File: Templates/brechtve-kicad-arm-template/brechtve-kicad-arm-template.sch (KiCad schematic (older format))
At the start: 16 parts, among them J1 DebugHeader_Cortex-M_SWD_UART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, J2 DebugHeader_Cortex-M_JTAG_10p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, J3 DebugHeader_UART_4p, SW1 SW_Push

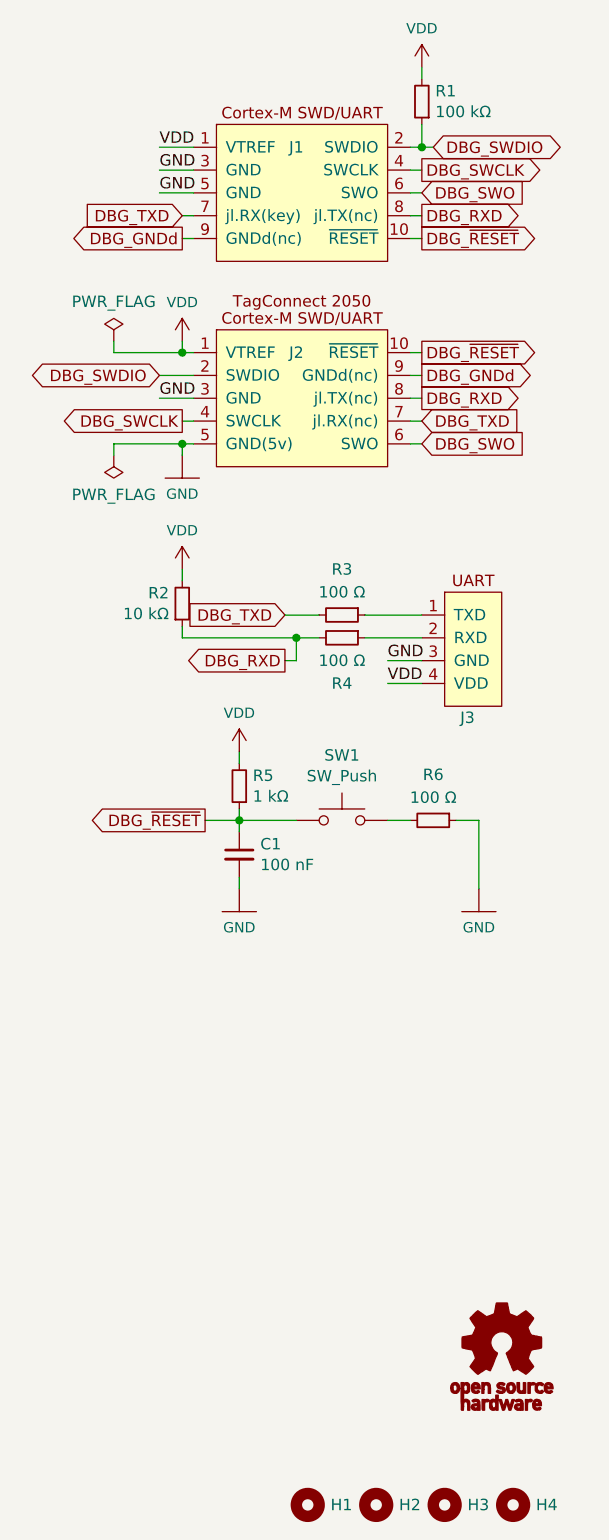
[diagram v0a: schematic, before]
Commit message: Modified schematic
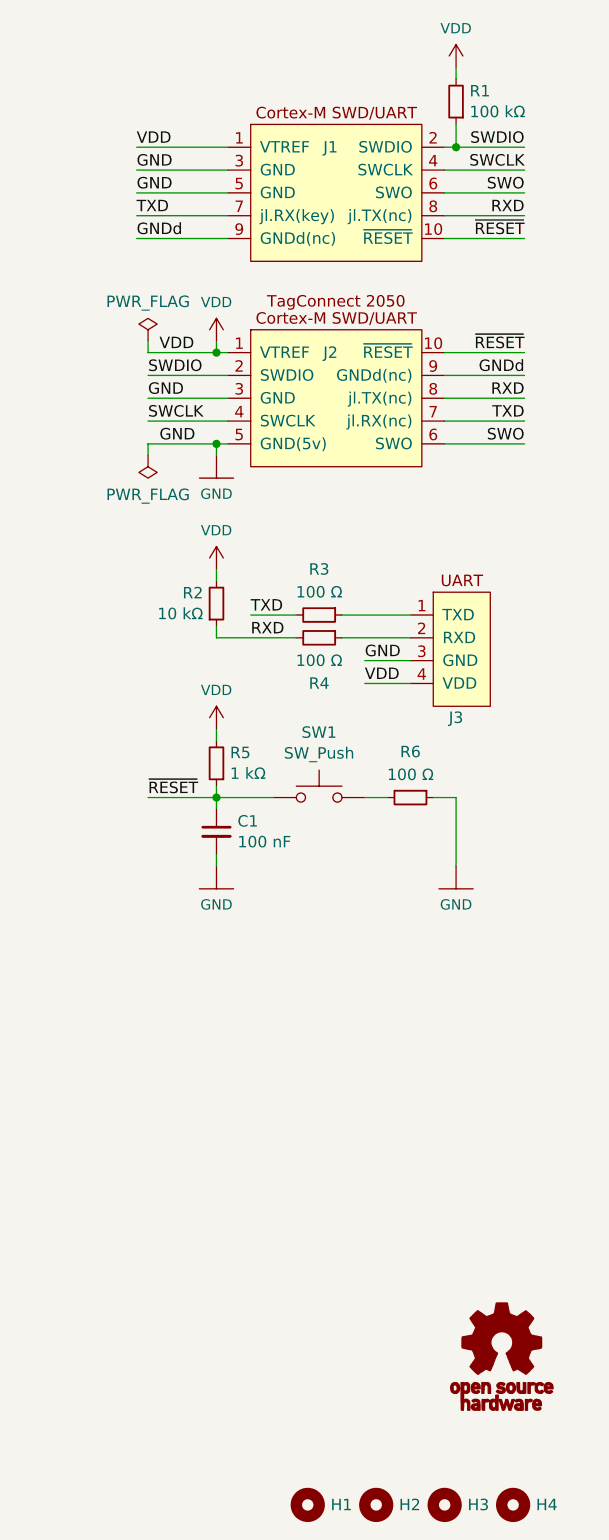
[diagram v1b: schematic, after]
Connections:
- net DBG_GNDd renamed GNDd
- net DBG_RXD renamed RXD
- net DBG_SWCLK renamed SWCLK
- net DBG_SWDIO renamed SWDIO
- net DBG_SWO renamed SWO
- net DBG_TXD renamed TXD
- net DBG_~RESET renamed ~RESET
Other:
- moved on the sheet: C1, J1, J2, J3, R1, R2, R3, R4, R5, R6, SW1
